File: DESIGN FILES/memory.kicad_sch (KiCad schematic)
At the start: 24 parts, among them J1 TF-15x15, U4 IS25WP064A-JBLE, U5 IS42S16160J-6BLI, U6 IRLML6401

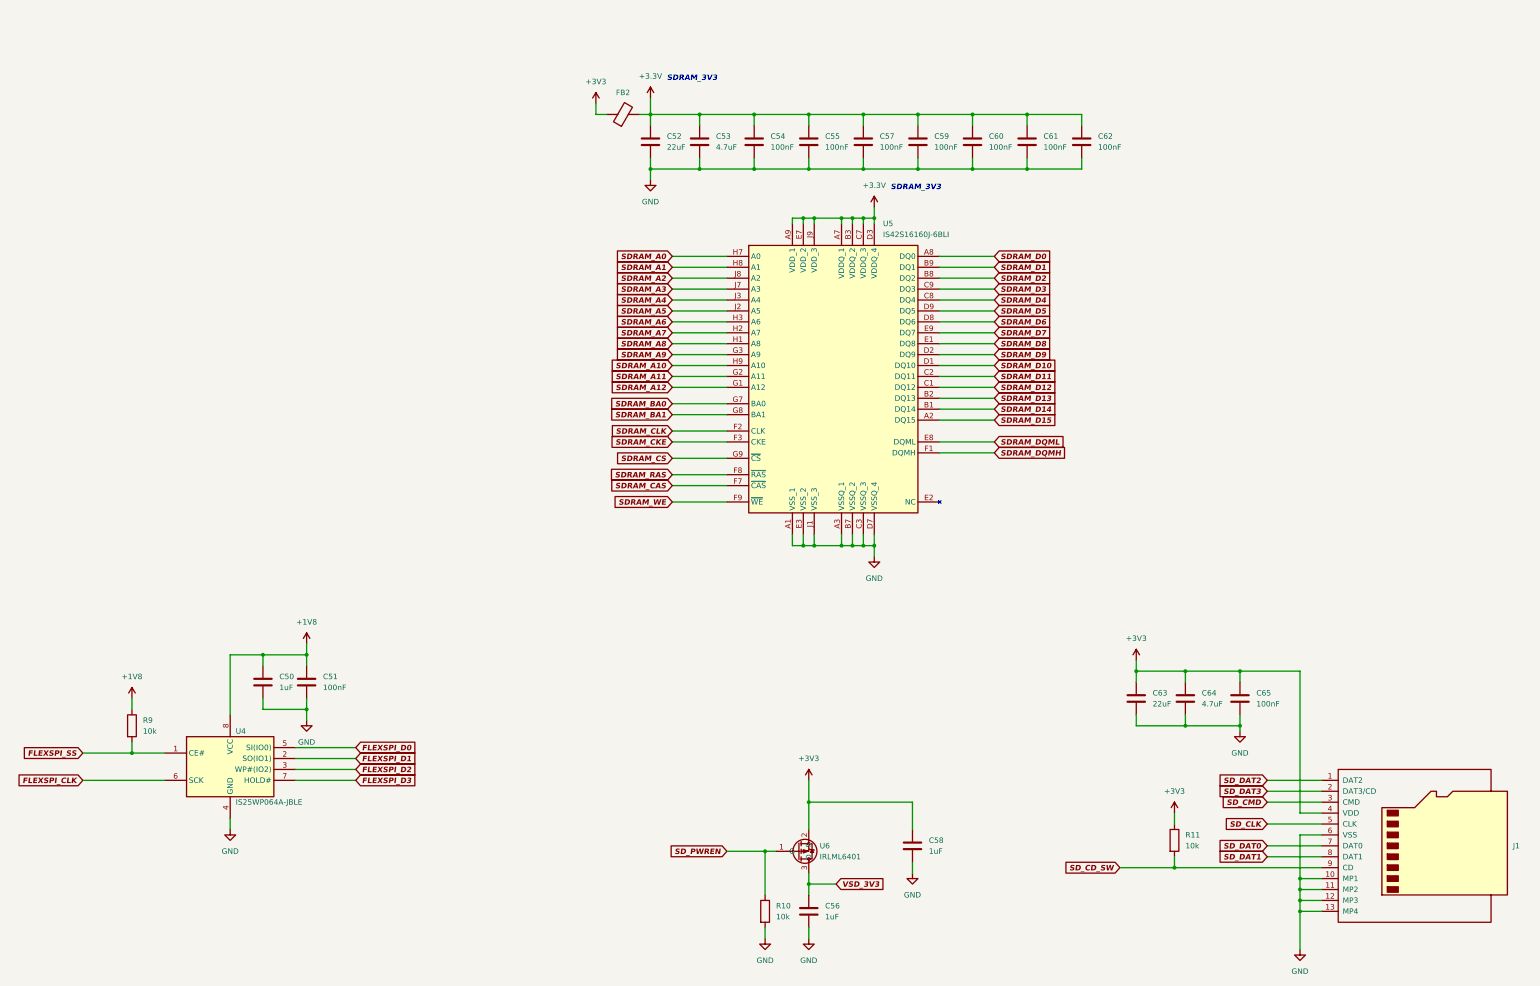
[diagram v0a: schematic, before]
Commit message: Refactoring schematic
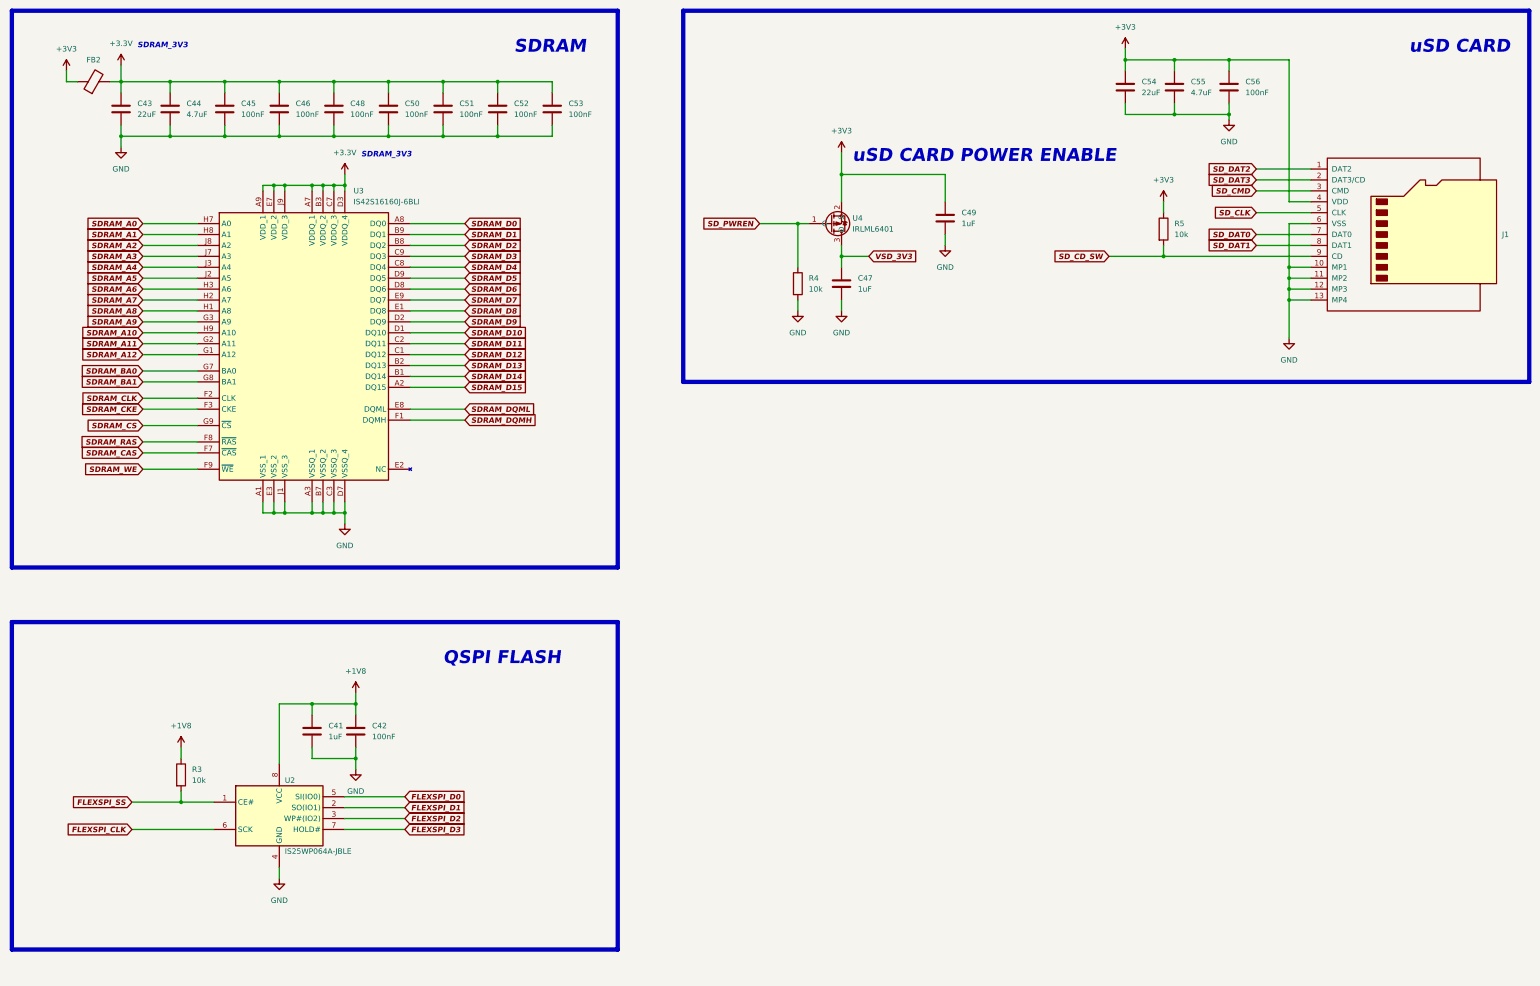
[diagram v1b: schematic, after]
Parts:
- renumbered C50 to C41, C51 to C42, C52 to C43, C53 to C44, C54 to C45, C55 to C46, C56 to C47, C57 to C48, C58 to C49, C59 to C50, C60 to C51, C61 to C52, C62 to C53, C63 to C54, C64 to C55, C65 to C56, R9 to R3, R10 to R4, R11 to R5, U4 to U2, U5 to U3, U6 to U4
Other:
- note added: "QSPI FLASH"
- note added: "SDRAM"
- note added: "uSD CARD"
- note added: "uSD CARD POWER ENABLE"
- moved on the sheet: C41, C42, C43, C44, C45, C46, C47, C48, C49, C50, C51, C52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
